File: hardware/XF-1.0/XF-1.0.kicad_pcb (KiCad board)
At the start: 2 copper layers, 144.8 x 99.7 mm, 23 parts, among them CN1 Conn_01x02, CN2 Conn_01x02, CN3 Conn_01x03, CN4 Conn_01x03, CN5 Conn_01x02, CN6 Conn_01x03, CN7 Conn_01x02

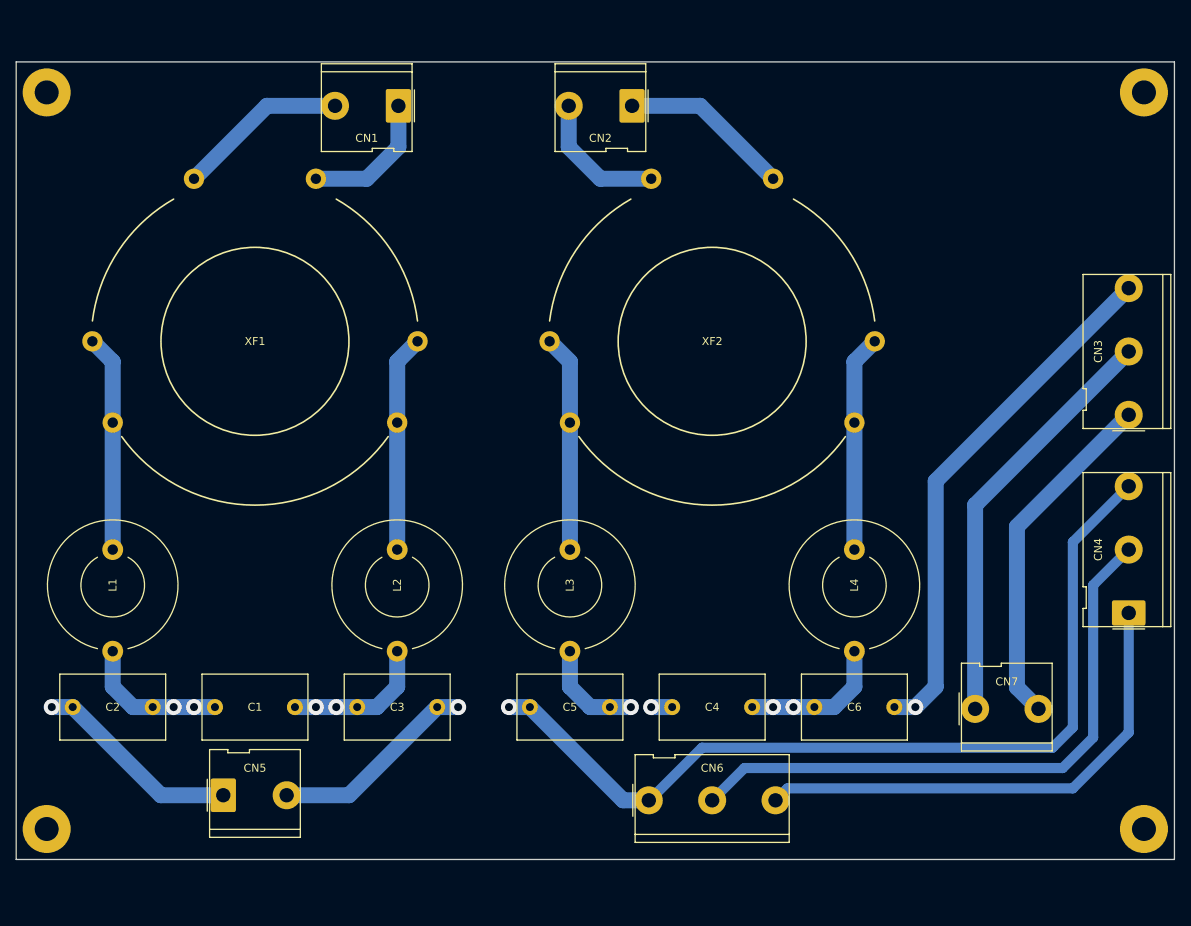
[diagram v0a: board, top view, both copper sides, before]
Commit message: modified:   README.md 	deleted:    hardware/CTL-1.0/CTL-1.0-backups/CTL-1.0-2025-05-28_203806.zip 	deleted:    hardware/CTL-1.0/CTL-1.0-backups/CTL-1.0-2025-05-28_204313.zip 	deleted:    hardware/CTL-1.0/CTL-1.0-backups/CTL-1.0-2025-05-30_173028.zip 	deleted:    hardware/CTL-1.0/CTL-1.0-backups/CTL-1.0-2025-05-30_174116.zip 	deleted:    hardware/CTL-1.0/CTL-1.0-backups/CTL-1.0-2025-05-30_175122.zip 	new file:   hardware/CTL-1.0/CTL-1.0-backups/CTL-1.0-2025-07-24_151142.zip 	new file:   hardware/CTL-1.0/CTL-1.0-backups/CTL-1.0-2025-07-24_172002.zip 	new file:   hardware/CTL-1.0/CTL-1.0-backups/CTL-1.0-2025-07-25_175122.zip 	new file:   hardware/CTL-1.0/CTL-1.0-backups/CTL-1.0-2025-07-26_120011.zip 	new file:   hardware/CTL-1.0/CTL-1.0-backups/CTL-1.0-2025-07-26_120808.zip 	modified:   hardware/CTL-1.0/CTL-1.0.kicad_pcb 	modified:   hardware/CTL-1.0/CTL-1.0.kicad_pro 	new file:   hardware/CTL-1.0/CTL-1.0.step 	deleted:    hardware/MSD-1.0/MSD-1.0-backups/MSD-1.0-2025-04-11_111943.zip 	deleted:    hardware/MSD-1.0/MSD-1.0-backups/MSD-1.0-2025-04-11_113401.zip 	new file:   hardware/MSD-1.0/MSD-1.0-backups/MSD-1.0-2025-07-25_163151.zip 	new file:   hardware/MSD-1.0/MSD-1.0-backups/MSD-1.0-2025-07-25_171843.zip 	modified:   hardware/MSD-1.0/MSD-1.0.kicad_pcb 	modified:   hardware/MSD-1.0/MSD-1.0.step 	new file:   hardware/MSD-1.1/MSD-1.1-backups/MSD-1.1-2025-07-24_151252.zip 	new file:   hardware/MSD-1.1/MSD-1.1-backups/MSD-1.1-2025-07-25_152939.zip 	new file:   hardware/MSD-1.1/MSD-1.1-backups/MSD-1.1-2025-07-25_162346.zip 	new file:   hardware/MSD-1.1/MSD-1.1-backups/MSD-1.1-2025-07-25_162917.zip 	modified:   hardware/MSD-1.1/MSD-1.1.kicad_pcb 	modified:   hardware/MSD-1.1/MSD-1.1.step 	modified:   hardware/MSD-1.1/fp-info-cache 	new file:   hardware/MSD-2.0/MSD-2.0-backups/MSD-2.0-2025-07-24_151230.zip 	deleted:    hardware/PS-2.0/PS-2.0-backups/PS-2.0-2025-05-07_010425.zip 	deleted:    hardware/PS-2.0/PS-2.0-backups/PS-2.0-2025-05-09_084820.zip 	deleted:    hardware/P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
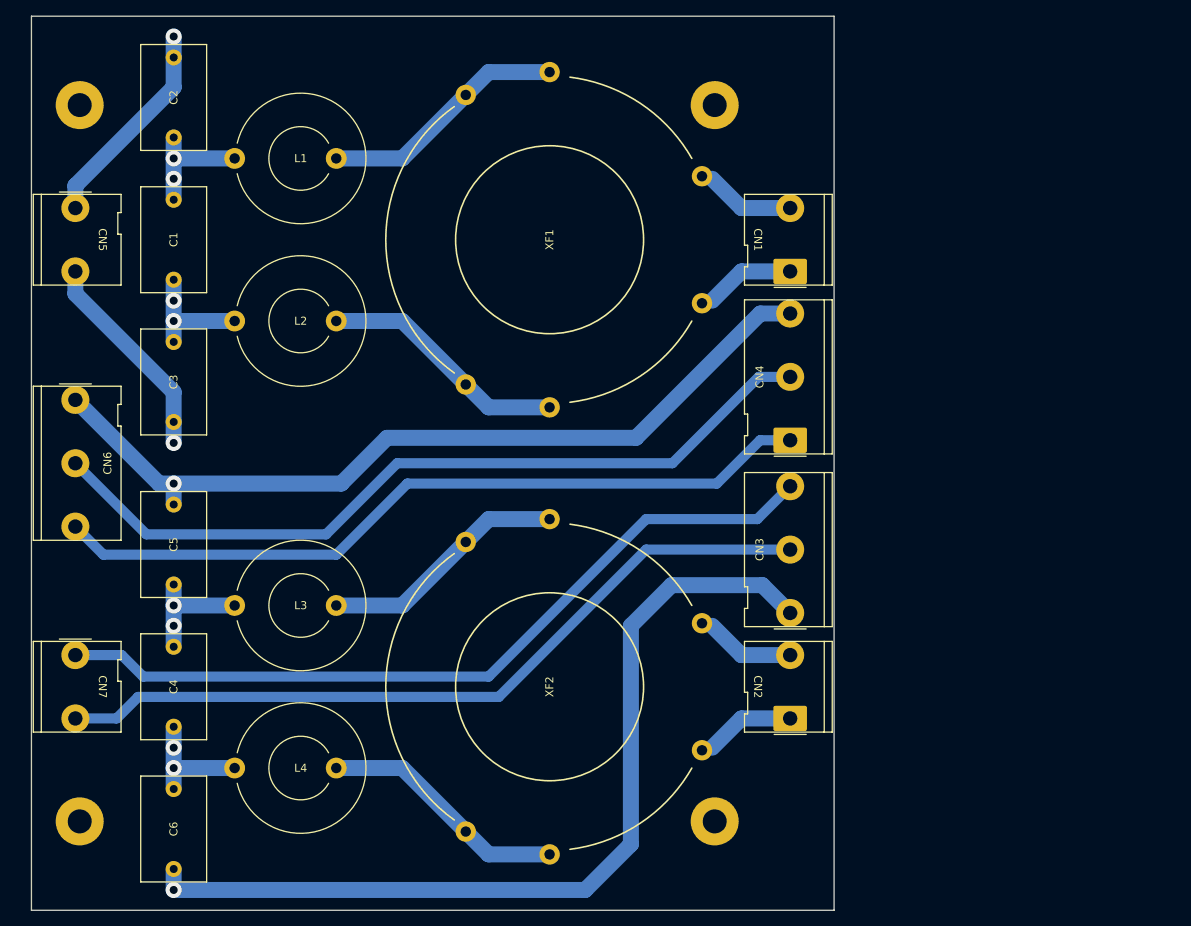
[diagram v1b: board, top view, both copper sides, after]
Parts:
- removed the H2 at (164.5, 50.2)
- added H3: ~, MountingHole:MountingHole_3mm_Pad, F.Cu at (110.8, 141.3)
- moved CN7 112.7 mm to (30.9, 120.5), turned to -90 degrees
- moved H4 105.2 mm to (110.8, 51.8)
- moved CN6 87.4 mm to (30.9, 88.6), turned to -90 degrees
- moved C6 80.7 mm to (43.2, 137.2), turned to -90 degrees
- moved CN2 79.1 mm to (120.2, 128.4), turned to 90 degrees
- moved CN5 75.7 mm to (30.9, 64.6), turned to -90 degrees
- moved L4 72.9 mm to (59.1, 134.6), turned to 180 degrees
- moved C2 71.2 mm to (43.2, 55.8), turned to 90 degrees
- moved C1 63.6 mm to (43.2, 63.6), turned to -90 degrees
- moved C4 62.8 mm to (43.2, 119.5), turned to -90 degrees
- moved L1 58.3 mm to (59.1, 58.4), turned to 180 degrees
- moved C5 56.6 mm to (43.2, 111.7), turned to 90 degrees
- moved CN1 53.2 mm to (120.2, 72.5), turned to 90 degrees
- moved C3 51.1 mm to (43.2, 81.4), turned to -90 degrees
- moved CN3 49.0 mm to (120.2, 115.2)
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- renumbered H3 to H2
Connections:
- C6 pad 2: Net-(CN3-Pin_3) -> Net-(CN3-Pin_1)
- CN7 pad 1: Net-(CN3-Pin_2) -> Net-(CN3-Pin_3)
- CN7 pad 2: Net-(CN3-Pin_1) -> Net-(CN3-Pin_2)
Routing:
- net Net-(CN3-Pin_1): track 43.7 -> 112.9 mm, vias 0 -> 1
- net Net-(CN3-Pin_2): track 52.6 -> 98.1 mm
- net Net-(CN3-Pin_3): track 66.0 -> 100.3 mm, vias 1 -> 0
- net Net-(CN4-Pin_1): track 62.6 -> 96.7 mm
- net Net-(CN4-Pin_2): track 76.2 -> 101.2 mm
- net Net-(CN1-Pin_2): track 21.4 -> 11.3 mm
- net Net-(CN2-Pin_1): track 21.4 -> 11.3 mm
- net Net-(CN4-Pin_3): track 112.1 -> 105.1 mm
- net Net-(CN2-Pin_2): track 17.1 -> 11.3 mm
- net Net-(CN1-Pin_1): track 17.1 -> 11.3 mm
- net Net-(L3-Pad1): track 27.1 -> 31.1 mm
- net Net-(L2-Pad1): track 27.1 -> 31.1 mm
- net Net-(L4-Pad1): track 27.1 -> 31.1 mm
- net Net-(L1-Pad1): track 27.1 -> 31.1 mm
- net Net-(C4-Pad2): track 18.3 -> 15.4 mm
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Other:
- board size 144.8 x 99.7 mm -> 100.3 x 111.8 mm
